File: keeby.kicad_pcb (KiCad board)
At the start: 2 copper layers, 292.1 x 116.2 mm, 192 parts, among them J1 Conn_01x04_Pin, J2 Conn_01x04_Pin, J3 JST_PH, J4 JST_PH, SW1 SW_Push, SW10 SW_Push, SW11 SW_Push, SW12 SW_Push, SW13 SW_Push, SW14 SW_Push, SW15 SW_Push, SW16 SW_Push, SW17 SW_Push, SW18 SW_Push, SW19 SW_Push, SW2 SW_Push, SW20 SW_Push, SW21 SW_Push, SW22 SW_Push, SW23 SW_Push, SW24 SW_Push, SW25 SW_Push, SW26 SW_Push, SW27 SW_Push, SW28 SW_Push, SW29 SW_Push, SW3 SW_Push, SW30 SW_Push, SW31 SW_Push, SW32 SW_Push, SW33 SW_Push, SW34 SW_Push, SW35 SW_Push, SW36 SW_Push, SW37 SW_Push, SW38 SW_Push, SW39 SW_Push, SW4 SW_Push, SW40 SW_Push, SW41 SW_Push, SW42 SW_Push, SW43 SW_Push, SW44 SW_Push, SW45 SW_Push, SW46 SW_Push, SW47 SW_Push, SW48 SW_Push, SW49 SW_Push, SW5 SW_Push, SW50 SW_Push, SW51 SW_Push, SW52 SW_Push, SW53 SW_Push, SW54 SW_Push, SW55 SW_Push, SW56 SW_Push, SW57 SW_Push, SW58 SW_Push, SW59 RotaryEncoder_Switch, SW6 SW_Push, SW60 RotaryEncoder_Switch, SW61 SW_SPDT, SW62 SW_SPDT, SW7 SW_Push, SW8 SW_Push, SW9 SW_Push, U3 SuperMini nRF52840, U4 SuperMini nRF52840

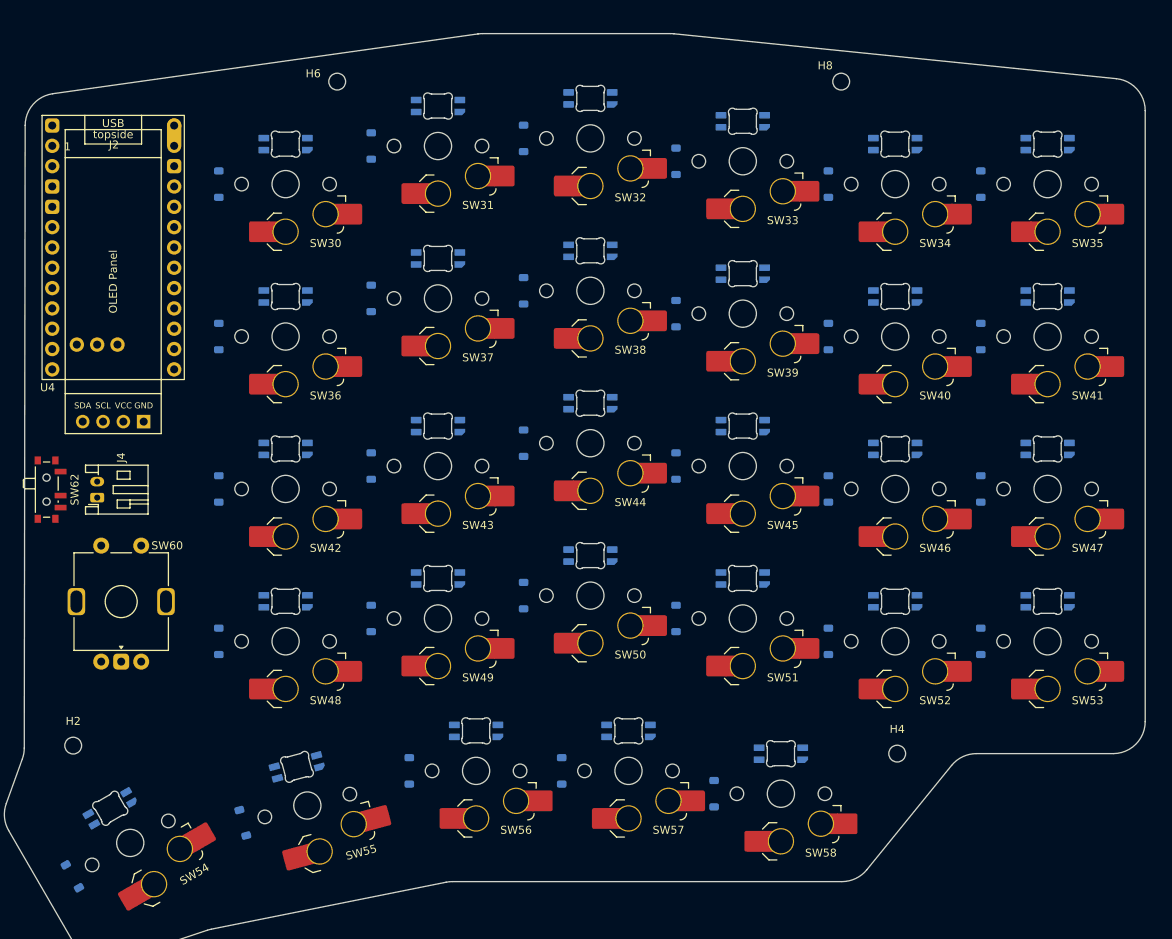
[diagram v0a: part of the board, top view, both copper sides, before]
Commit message: routed
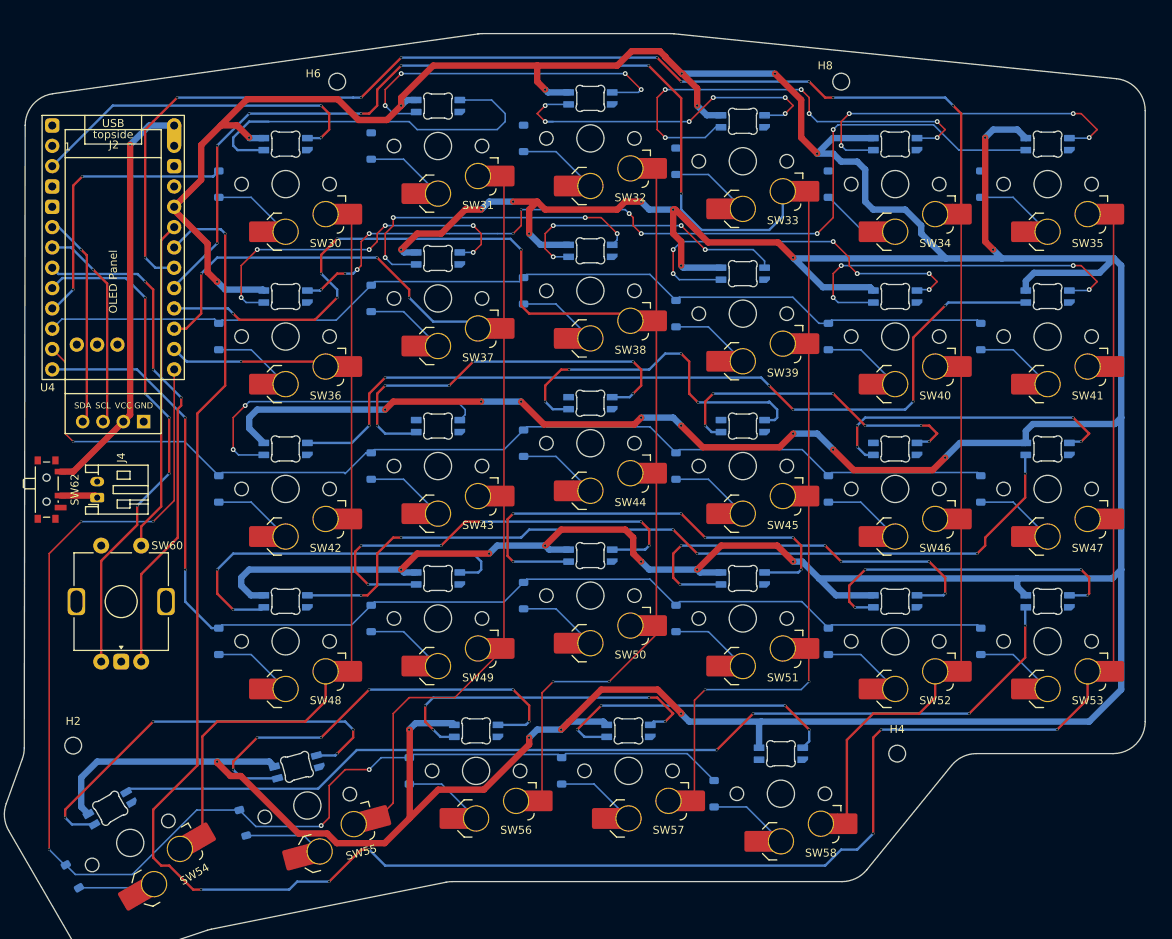
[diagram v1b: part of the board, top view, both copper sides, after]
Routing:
- net +3.3V: track 748.5 -> 1595.4 mm, vias 0 -> 37
- net COL6: track 84.6 -> 371.6 mm, vias 1 -> 8
- net COL5: track 154.3 -> 379.7 mm, vias 1 -> 10
- net COL4: track 170.2 -> 375.9 mm, vias 5 -> 14
- net ROW5: track 154.9 -> 323.1 mm, vias 4 -> 9
- net COL3: track 177.4 -> 342.6 mm, vias 7 -> 14
- net ROW4: track 152.1 -> 300.8 mm, vias 0 -> 2
- net COL2: track 225.1 -> 363.9 mm, vias 5 -> 8
- net ROW3: track 129.6 -> 263.4 mm, vias 2 -> 3
- net Net-(L53-DOUT): track 0.00 -> 125.7 mm, vias 0 -> 4
- net ROW2: track 123.2 -> 245.7 mm
- net Net-(L35-DOUT): track 0.00 -> 112.1 mm, vias 0 -> 10
- net COL1: track 279.8 -> 390.2 mm, vias 3 -> 4
- net Net-(L41-DOUT): track 0.00 -> 107.4 mm, vias 0 -> 6
- net Net-(L47-DOUT): track 0.00 -> 105.6 mm, vias 0 -> 6
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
